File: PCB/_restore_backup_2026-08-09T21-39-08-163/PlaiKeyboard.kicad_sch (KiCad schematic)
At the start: 177 parts, among them SW1 SW_Push_45deg, SW10 SW_Push_45deg, SW11 SW_Push_45deg, SW12 SW_Push_45deg, SW13 SW_Push_45deg, SW14 SW_Push_45deg, SW15 RotaryEncoder_Switch, SW16 SW_Push_45deg, SW17 SW_Push_45deg, SW18 SW_Push_45deg, SW19 SW_Push_45deg, SW2 SW_Push_45deg, SW20 SW_Push_45deg, SW21 SW_Push_45deg, SW22 SW_Push_45deg, SW23 SW_Push_45deg, SW24 SW_Push_45deg, SW25 SW_Push_45deg, SW26 SW_Push_45deg, SW27 SW_Push_45deg, SW28 SW_Push_45deg, SW29 SW_Push_45deg, SW3 SW_Push_45deg, SW30 SW_Push_45deg, SW31 SW_Push_45deg, SW32 SW_Push_45deg, SW33 SW_Push_45deg, SW34 SW_Push_45deg, SW35 SW_Push_45deg, SW36 SW_Push_45deg, SW37 SW_Push_45deg, SW38 SW_Push_45deg, SW39 SW_Push_45deg, SW4 SW_Push_45deg, SW40 SW_Push_45deg, SW41 SW_Push_45deg, SW42 SW_Push_45deg, SW43 SW_Push_45deg, SW44 SW_Push_45deg, SW45 SW_Push_45deg, SW46 SW_Push_45deg, SW47 SW_Push_45deg, SW48 SW_Push_45deg, SW49 SW_Push_45deg, SW5 SW_Push_45deg, SW50 SW_Push_45deg, SW51 SW_Push_45deg, SW52 SW_Push_45deg, SW53 SW_Push_45deg, SW54 SW_Push_45deg, SW55 SW_Push_45deg, SW56 SW_Push_45deg, SW57 SW_Push_45deg, SW58 SW_Push_45deg, SW59 SW_Push_45deg, SW6 SW_Push_45deg, SW60 SW_Push_45deg, SW61 SW_Push_45deg, SW62 SW_Push_45deg, SW63 SW_Push_45deg, SW64 SW_Push_45deg, SW65 SW_Push_45deg, SW66 SW_Push_45deg, SW67 SW_Push_45deg, SW68 SW_Push_45deg, SW69 SW_Push_45deg, SW7 SW_Push_45deg, SW70 SW_Push_45deg, SW71 SW_Push_45deg, SW72 SW_Push_45deg, SW73 SW_Push_45deg, SW74 SW_Push_45deg, SW75 SW_Push_45deg, SW76 SW_Push_45deg, SW77 SW_Push_45deg, SW78 SW_Push_45deg, SW79 SW_Push_45deg, SW8 SW_Push_45deg, SW80 SW_Push_45deg, SW81 SW_Push_45deg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

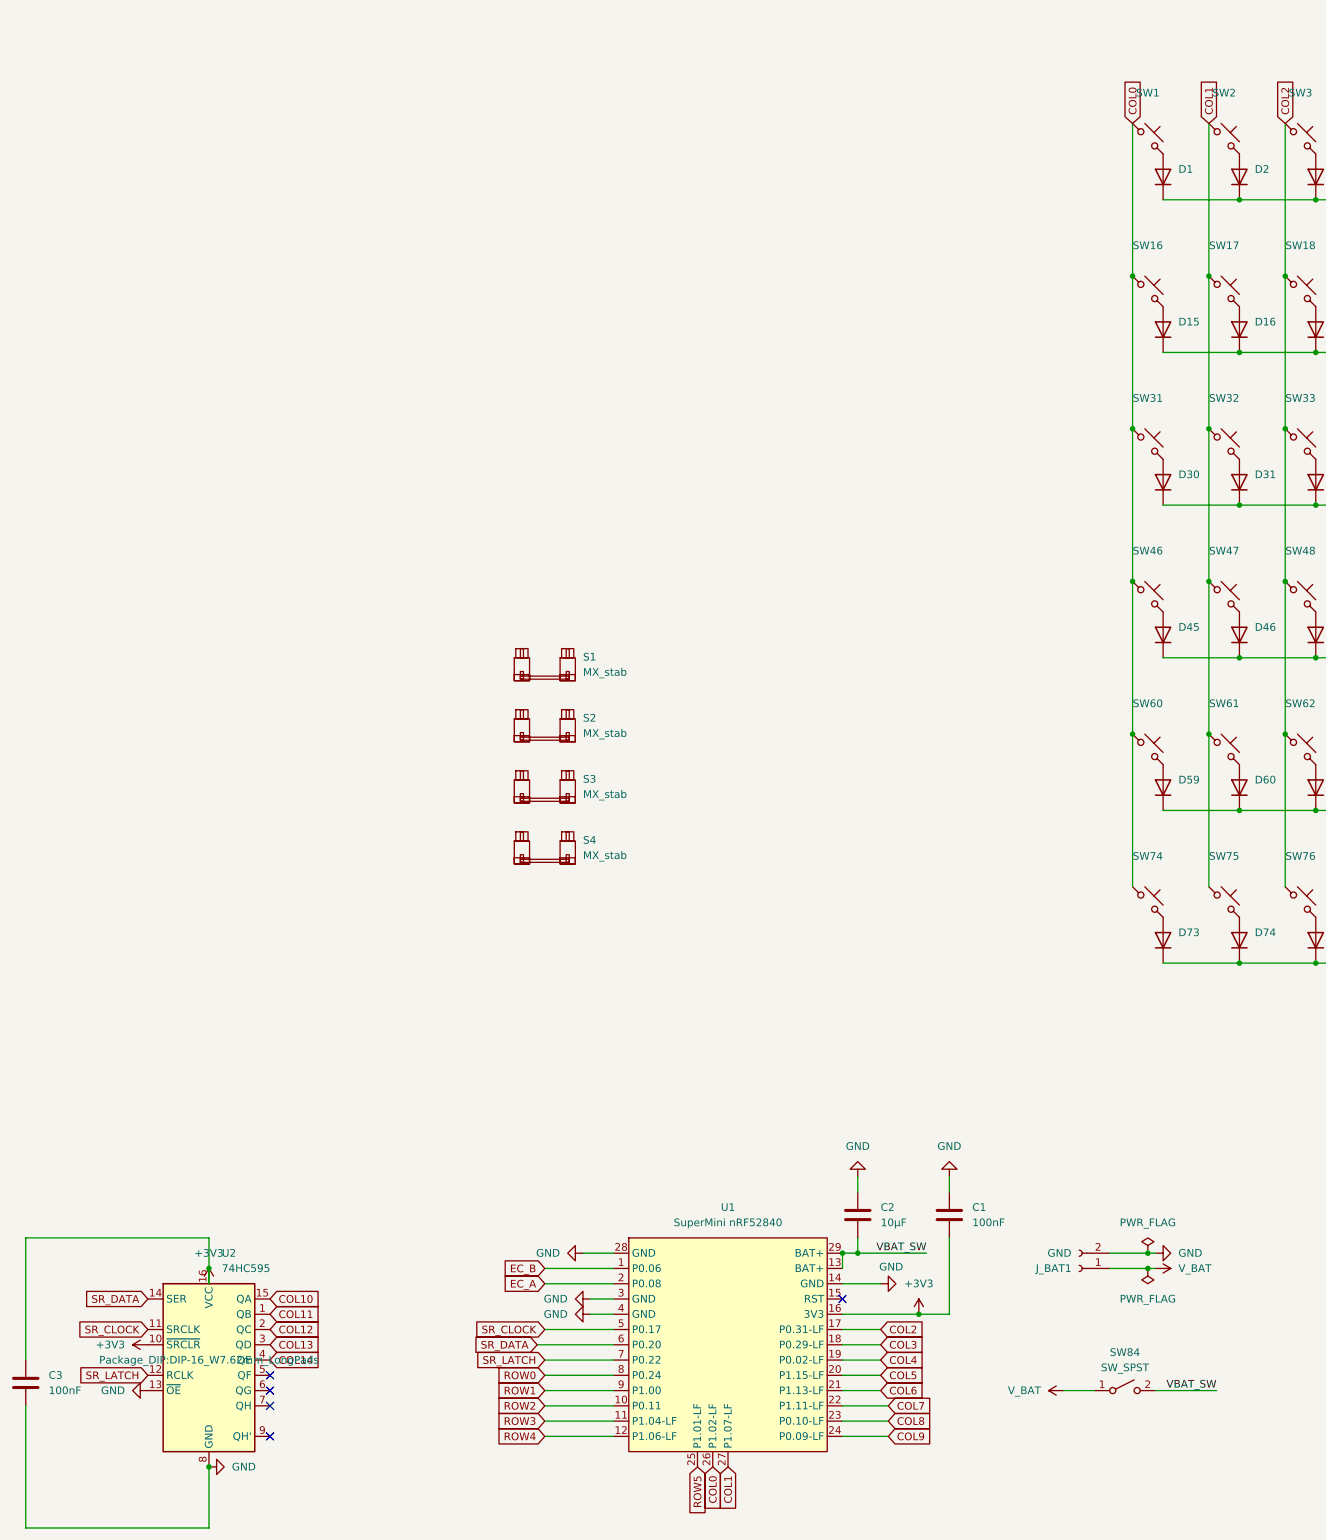
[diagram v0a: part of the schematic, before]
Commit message: ACTUALLY FINISHED WITH THE PCB
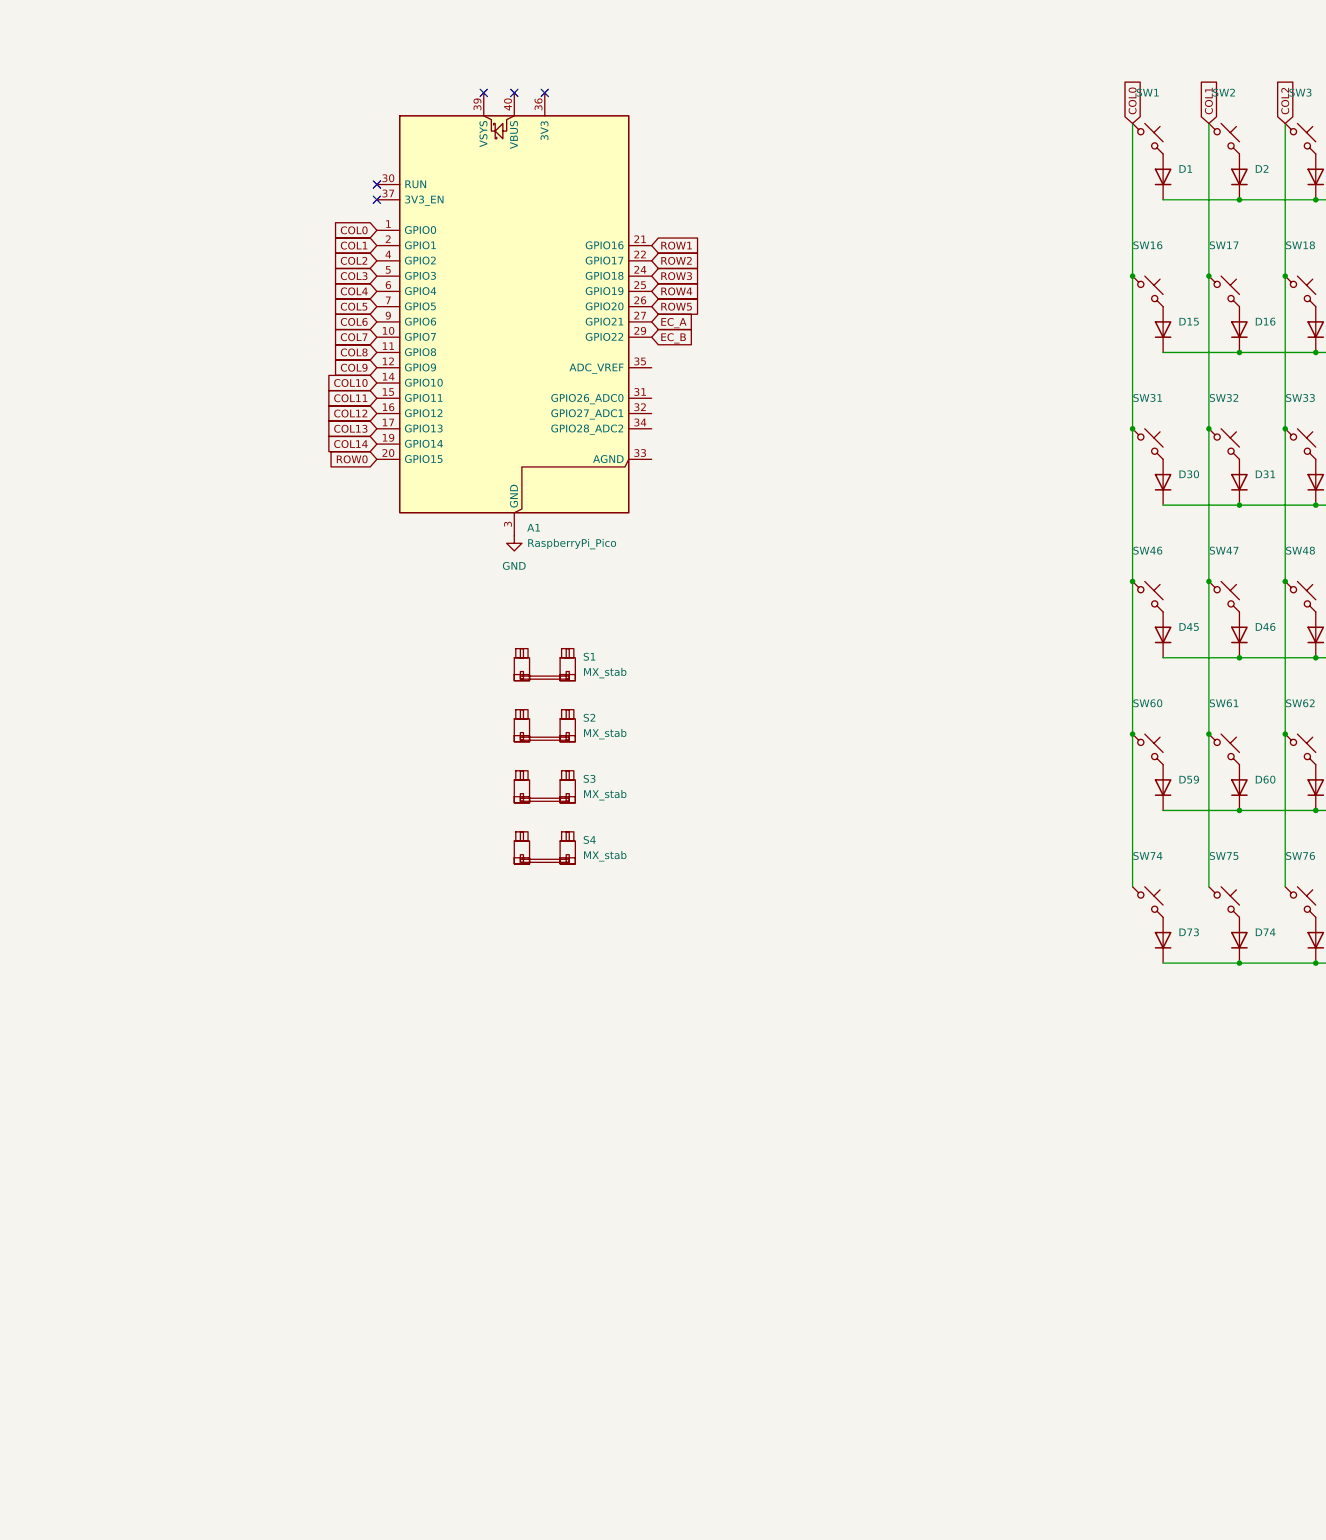
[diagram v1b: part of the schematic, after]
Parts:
- removed C1, C3: 100nF, Capacitor_THT:C_Rect_L11.5mm_W5.2mm_P10.00mm_MKT, symbol Device:C
- removed C2: 10µF, Capacitor_THT:C_Disc_D4.7mm_W2.5mm_P5.00mm, symbol Device:C
- removed J_BAT1: GND, Connector_JST:JST_PH_S2B-PH-K_1x02_P2.00mm_Horizontal, symbol Connector:Conn_01x02_Socket
- removed SW84: SW_SPST, microChave:1P2T_SS-12D00_CNK, symbol Switch:SW_SPST
- removed U1: SuperMini nRF52840, PCM_marbastlib-xp-promicroish:SuperMini_nRF52840_AH_USBup, symbol marbastlib-promicroish:SuperMini_nRF52840
- removed U2: 74HC595, Package_DIP:DIP-16_W7.62mm_LongPads, symbol 74xx:74HC595
- added A1: RaspberryPi_Pico, Module:RaspberryPi_Pico_Common_Unspecified, symbol MCU_Module:RaspberryPi_Pico
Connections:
- net COL0: now also A1.1 (GPIO0)
- net COL1: now also A1.2 (GPIO1)
- net COL10: now also A1.14 (GPIO10)
- net COL11: now also A1.15 (GPIO11)
- net COL12: now also A1.16 (GPIO12)
- net COL13: now also A1.17 (GPIO13)
- net COL14: now also A1.19 (GPIO14)
- net COL2: now also A1.4 (GPIO2)
- net COL3: now also A1.5 (GPIO3)
- net COL4: now also A1.6 (GPIO4)
- net COL5: now also A1.7 (GPIO5)
- net COL6: now also A1.9 (GPIO6)
- net COL7: now also A1.10 (GPIO7)
- net COL8: now also A1.11 (GPIO8)
- net COL9: now also A1.12 (GPIO9)
- net EC_A: now also A1.27 (GPIO21)
- net EC_B: now also A1.29 (GPIO22)
- net GND: now also A1.13 (GND), A1.18 (GND), A1.23 (GND), A1.28 (GND), A1.3 (GND), A1.38 (GND), A1.8 (GND)
- net ROW0: now also A1.20 (GPIO15)
- net ROW1: now also A1.21 (GPIO16)
- net ROW2: now also A1.22 (GPIO17)
- net ROW3: now also A1.24 (GPIO18)
- net ROW4: now also A1.25 (GPIO19)
- net ROW5: now also A1.26 (GPIO20)
